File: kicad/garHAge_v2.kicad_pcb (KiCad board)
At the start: 2 copper layers, 99 x 77 mm, 77 parts, among them J1 0813-1X1T-57-F, J2 Serial Interface, J3 SJ1-2503A, J4 SJ1-2503A, J5 SJ1-2503A, J6 SJ1-2503A, J7 SJ1-2503A, J8 SJ1-2503A, K1 G5LE-14_DC3, K2 G5LE-14_DC3, K3 G5LE-14_DC3, Q1 BC846B_215, Q2 BC846B_215, Q3 BC846B_215, U1 ATMEGA328P-AU, U2 NCP1090, U3 PG02S4805A, U4 W5500, U5 LTV-817S, U6 LTV-817S, U7 LTV-817S, X1 ICSP, X2 SPI Disconnect, Y1 8MHz, Y2 25MHz

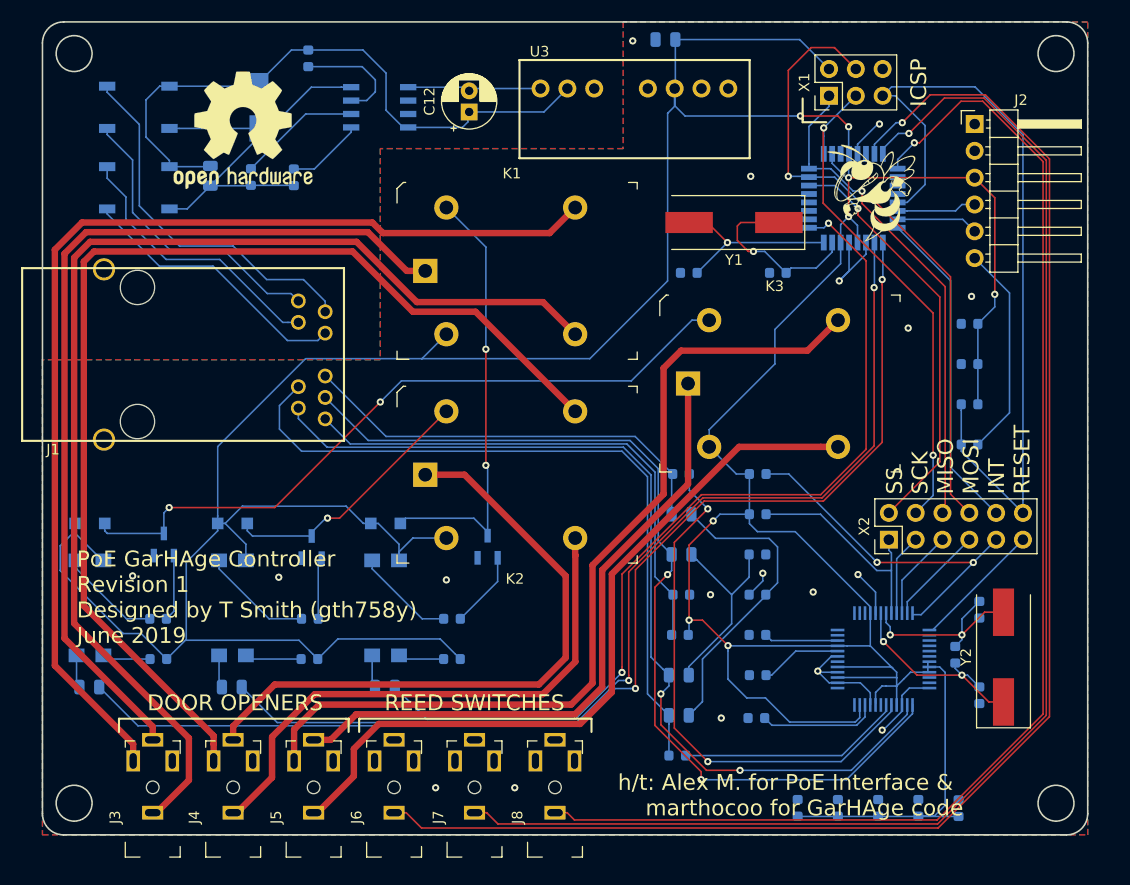
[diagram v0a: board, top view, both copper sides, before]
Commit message: Add files via upload
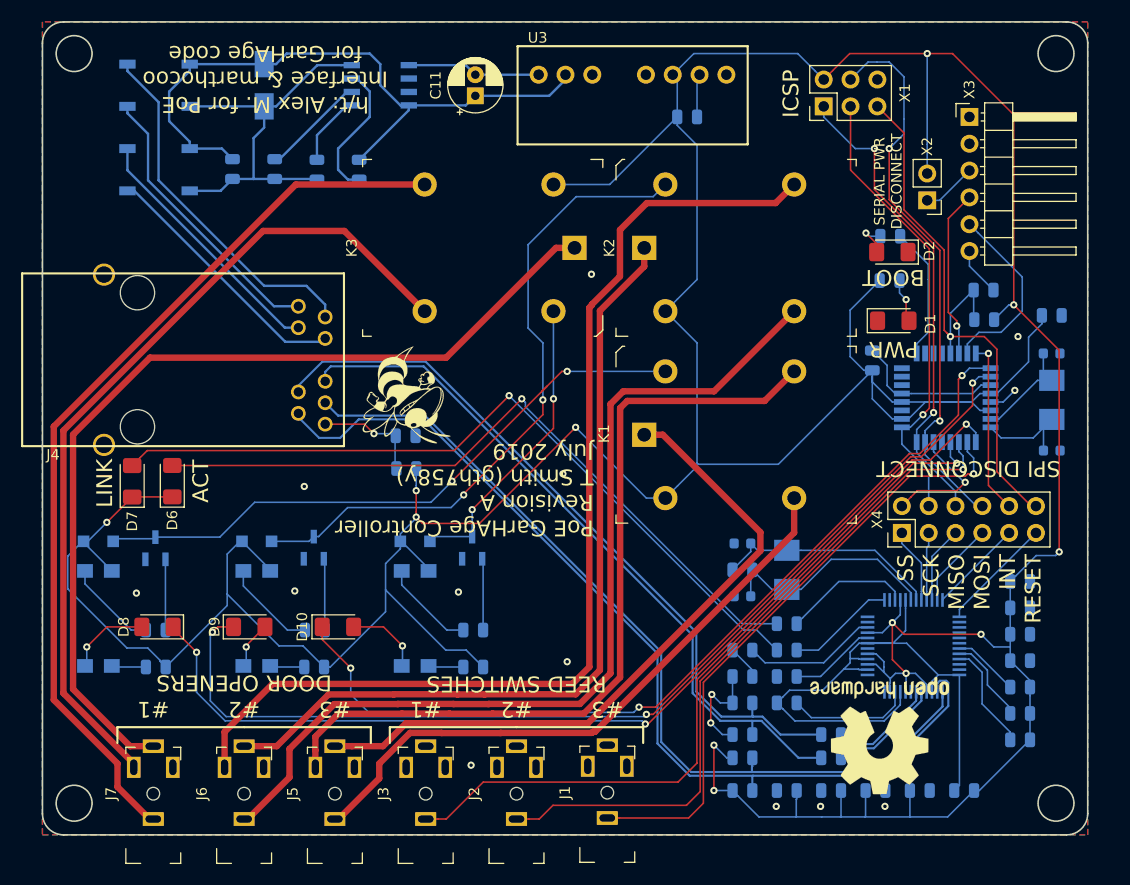
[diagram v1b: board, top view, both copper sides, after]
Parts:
- removed J8: SJ1-2503A, digikey-footprints:Headphone_Jack_2.5mm_SJ1-2503A
- added C23: 4.7u, Capacitor_SMD:C_0805_2012Metric, B.Cu at (191.5, 103.0)
- added C24: 18p, Capacitor_SMD:C_0603_1608Metric, B.Cu at (187.3, 95.4)
- added C25: 18p, Capacitor_SMD:C_0603_1608Metric, B.Cu at (187.3, 90.4)
- added D10: LED, LED_SMD:LED_1206_3216Metric_Pad1.42x1.75mm_HandSolder, F.Cu at (149.0, 98.3)
- added D11: CGRKM4007-HF, Diode_SMD:D_SOD-123F, B.Cu at (126.3, 90.2)
- added D12: CGRKM4007-HF, Diode_SMD:D_SOD-123F, B.Cu at (141.3, 90.2)
- added D13: CGRKM4007-HF, Diode_SMD:D_SOD-123F, B.Cu at (156.3, 90.2)
- added R19: 100, Resistor_SMD:R_0805_2012Metric, B.Cu at (146.7, 102.1)
- added R20: 100, Resistor_SMD:R_0805_2012Metric, B.Cu at (161.8, 102.1)
- added R21: 1k, Resistor_SMD:R_0805_2012Metric, B.Cu at (131.7, 98.6)
- added R22: 1k, Resistor_SMD:R_0805_2012Metric, B.Cu at (146.8, 98.6)
- added R23: 1k, Resistor_SMD:R_0805_2012Metric, B.Cu at (161.8, 98.6)
- added X3: Serial Interface, Connector_PinHeader_2.54mm:PinHeader_1x06_P2.54mm_Horizontal, F.Cu at (208.8, 50.0)
- added X4: SPI Disconnect, Connector_PinHeader_2.54mm:PinHeader_2x06_P2.54mm_Vertical, F.Cu at (202.4, 89.4)
- C1, C2: value 10n -> 6.8n; footprint Capacitor_SMD:C_0603_1608Metric -> Capacitor_SMD:C_0805_2012Metric
- C10, C15, C16, C17, C18, C9, L1: footprint Capacitor_SMD:C_0603_1608Metric -> Capacitor_SMD:C_0805_2012Metric
- C11: value 100n -> 22u; footprint Capacitor_SMD:C_0805_2012Metric -> Capacitor_THT:CP_Radial_D5.0mm_P2.00mm; moved to F.Cu
- C12: value 22u -> 10u; footprint Capacitor_THT:CP_Radial_D5.0mm_P2.00mm -> Capacitor_SMD:C_0805_2012Metric; moved to B.Cu
- C13: value 10u -> 10u/16V
- C14: value 100n -> 10u/16V; footprint Capacitor_SMD:C_0603_1608Metric -> Capacitor_SMD:C_0805_2012Metric
- C19: value 10n -> 100n; footprint Capacitor_SMD:C_0603_1608Metric -> Capacitor_SMD:C_0805_2012Metric
- C20: value 4.7u -> 100n; footprint Capacitor_SMD:C_0603_1608Metric -> Capacitor_SMD:C_0805_2012Metric
- C21, C7, C8: value 18p -> 100n; footprint Capacitor_SMD:C_0603_1608Metric -> Capacitor_SMD:C_0805_2012Metric
- C22: value 18p -> 10n; footprint Capacitor_SMD:C_0603_1608Metric -> Capacitor_SMD:C_0805_2012Metric
- C3: value 100n -> 22n; footprint Capacitor_SMD:C_0603_1608Metric -> Capacitor_SMD:C_0805_2012Metric
- C4: value 100n -> 10n; footprint Capacitor_SMD:C_0603_1608Metric -> Capacitor_SMD:C_0805_2012Metric
- C5, C6: value 100n -> 18p
- D1, D2: value MDB6S -> LED; footprint tyler_components:Micro-DIP-4 -> LED_SMD:LED_1206_3216Metric_Pad1.42x1.75mm_HandSolder; moved to F.Cu
- D3: value SMAJ58A -> MDB6S; footprint Diode_SMD:D_SMA -> tyler_components:Micro-DIP-4
- D4: value LED -> MDB6S; footprint LED_SMD:LED_0805_2012Metric -> tyler_components:Micro-DIP-4
- D5: value LED -> SMAJ58A; footprint LED_SMD:LED_0805_2012Metric -> Diode_SMD:D_SMA
- D6: footprint LED_SMD:LED_0805_2012Metric -> LED_SMD:LED_1206_3216Metric_Pad1.42x1.75mm_HandSolder; moved to F.Cu
- D7, D8, D9: value CGRKM4007-HF -> LED; footprint Diode_SMD:D_SOD-123F -> LED_SMD:LED_1206_3216Metric_Pad1.42x1.75mm_HandSolder; moved to F.Cu
- J1: value 0813-1X1T-57-F -> SJ1-2503A; footprint tyler_components:0813-1X1T-57-F_RJ45-Jack -> digikey-footprints:Headphone_Jack_2.5mm_SJ1-2503A
- J2: value Serial Interface -> SJ1-2503A; footprint Connector_PinHeader_2.54mm:PinHeader_1x06_P2.54mm_Horizontal -> digikey-footprints:Headphone_Jack_2.5mm_SJ1-2503A
- J4: value SJ1-2503A -> 0813-1X1T-57-F; footprint digikey-footprints:Headphone_Jack_2.5mm_SJ1-2503A -> tyler_components:0813-1X1T-57-F_RJ45-Jack
- R10: value 10k -> 4420; footprint Resistor_SMD:R_0603_1608Metric -> Resistor_SMD:R_0805_2012Metric
- R11: footprint Resistor_SMD:R_0603_1608Metric -> Resistor_SMD:R_0805_2012Metric
- R12: value 1M -> 10k; footprint Resistor_SMD:R_0603_1608Metric -> Resistor_SMD:R_0805_2012Metric
- R13: value 1k -> 10k; footprint Resistor_SMD:R_0603_1608Metric -> Resistor_SMD:R_0805_2012Metric
- R14: value 1k -> 12.4k; footprint Resistor_SMD:R_0603_1608Metric -> Resistor_SMD:R_0805_2012Metric
- R15: value 1k -> 1M; footprint Resistor_SMD:R_0603_1608Metric -> Resistor_SMD:R_0805_2012Metric
- R16, R17: value 510 -> 330; footprint Resistor_SMD:R_0603_1608Metric -> Resistor_SMD:R_0805_2012Metric
- R18: value 510 -> 100; footprint Resistor_SMD:R_0603_1608Metric -> Resistor_SMD:R_0805_2012Metric
- R5: value 12k -> 330; footprint Resistor_SMD:R_0603_1608Metric -> Resistor_SMD:R_0805_2012Metric
- R6: value 24.9k -> 12k; footprint Resistor_SMD:R_0603_1608Metric -> Resistor_SMD:R_0805_2012Metric
- R7: value 178k -> 330; footprint Resistor_SMD:R_0603_1608Metric -> Resistor_SMD:R_0805_2012Metric
- R8: value 4420 -> 24.9k; footprint Resistor_SMD:R_0603_1608Metric -> Resistor_SMD:R_0805_2012Metric
- R9: value 12.4k -> 178k; footprint Resistor_SMD:R_0603_1608Metric -> Resistor_SMD:R_0805_2012Metric
- X2: value SPI Disconnect -> Serial Pwr Disconnect; footprint Connector_PinHeader_2.54mm:PinHeader_2x06_P2.54mm_Vertical -> Connector_PinHeader_2.54mm:PinHeader_1x02_P2.54mm_Vertical
- Y1, Y2: footprint Crystal:Crystal_SMD_HC49-SD -> Crystal:Crystal_SMD_5032-2Pin_5.0x3.2mm; moved to B.Cu
- moved REF** 83.2 mm to (200.3, 108.6), turned to 180 degrees
- moved J2 76.9 mm to (165.9, 114.1), turned to 90 degrees
- moved D2 72.7 mm to (201.5, 62.8), turned to 180 degrees
- moved D1 72.6 mm to (201.6, 69.3), turned to 0 degrees
- moved C10 72.2 mm to (139.0, 54.9), turned to 270 degrees
- moved R6 68.6 mm to (210.2, 69.2), turned to 0 degrees
- moved R9 66.6 mm to (147.0, 55.0), turned to 270 degrees
- moved C13 61.3 mm to (213.6, 94.0), turned to 0 degrees
- moved D4 60.9 mm to (132.0, 47.0), turned to 270 degrees
- moved J1 60.8 mm to (174.5, 114.0)
- moved D5 57.1 mm to (142.0, 47.0), turned to 270 degrees
- moved R7 56.8 mm to (201.3, 61.3), turned to 180 degrees
- moved R10 56.2 mm to (143.0, 54.9), turned to 270 degrees
- moved R15 56.0 mm to (187.3, 92.9), turned to 180 degrees
- moved R13 53.9 mm to (213.6, 104.0), turned to 180 degrees
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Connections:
- C1 pad 2: Net-(C1-Pad2) -> /RD-
- C10 pad 1: +3V3 -> Net-(C10-Pad1)
- C10 pad 2: GND -> Net-(C10-Pad2)
- C11 pad 1: Net-(C11-Pad1) -> Net-(C10-Pad1)
- C12 pad 1: Net-(C11-Pad1) -> +3V3
- C12 pad 2: Net-(C12-Pad2) -> GND
- C19 pad 1: Net-(C19-Pad1) -> +3V3
- C2 pad 2: Net-(C2-Pad2) -> /RD+
- C20 pad 1: Net-(C20-Pad1) -> +3V3
- C21 pad 1: GND -> +3V3
- C21 pad 2: Net-(C21-Pad2) -> GND
- C22 pad 1: GND -> Net-(C22-Pad1)
- C22 pad 2: Net-(C22-Pad2) -> GND
- C3 pad 2: Net-(C3-Pad2) -> /CT
- C6 pad 1: DTR -> Net-(C6-Pad1)
- C6 pad 2: RESET -> GND
- C7 pad 1: GND -> DTR
- C7 pad 2: Net-(C7-Pad2) -> RESET
- C8 pad 1: Net-(C8-Pad1) -> +3V3
- D1 pad 1: Net-(C11-Pad1) -> GND
- D1 pad 2: Net-(C11-Pad2) -> Net-(D1-Pad2)
- D2 pad 1: Net-(C11-Pad1) -> GND
- D2 pad 2: Net-(C11-Pad2) -> /BOOT_STATUS
- D3 pad 1: Net-(C11-Pad1) -> Net-(C10-Pad1)
- D3 pad 2: Net-(C11-Pad2) -> Net-(C10-Pad2)
- D4 pad 1: D1RELAY -> Net-(C10-Pad1)
- D4 pad 2: Net-(D4-Pad2) -> Net-(C10-Pad2)
- D5 pad 1: D2RELAY -> Net-(C10-Pad1)
- D5 pad 2: Net-(D5-Pad2) -> Net-(C10-Pad2)
- D6 pad 1: D3RELAY -> +3V3
- D8 pad 1: +3V3 -> D1RELAY
- D9 pad 1: +3V3 -> D2RELAY
- J1 pad 1: /W5100_Ethernet_Interface/TD+ -> D1SENSOR
- J1 pad 2: Net-(C2-Pad2) -> (no net)
- J2 pad 1: GND -> D2SENSOR
- J2 pad 2: GND -> (no net)
- J2 pad 3: +3V3 -> (no net)
- J2 pad 4: RXI -> GND
- J3 pad 1: Net-(J3-Pad1) -> D3SENSOR
- J3 pad 3: Net-(J3-Pad3) -> (no net)
- J3 pad 4: Net-(J3-Pad4) -> GND
- J4 pad 1: Net-(J4-Pad1) -> /W5100_Ethernet_Interface/TD+
- J4 pad 2: (no net) -> /RD+
- J6 pad 3: (no net) -> Net-(J6-Pad3)
- J6 pad 4: GND -> Net-(J6-Pad4)
- J7 pad 3: (no net) -> Net-(J7-Pad3)
- J7 pad 4: GND -> Net-(J7-Pad4)
- K1 pad 1: Net-(J3-Pad4) -> Net-(J5-Pad4)
- K1 pad 3: Net-(J3-Pad1) -> Net-(J5-Pad1)
- K1 pad 4: Net-(J3-Pad3) -> Net-(J5-Pad3)
- K1 pad 5: Net-(D7-Pad2) -> Net-(D11-Pad2)
- K2 pad 1: Net-(J4-Pad4) -> Net-(J6-Pad4)
- K2 pad 3: Net-(J4-Pad1) -> Net-(J6-Pad1)
- K2 pad 4: Net-(J4-Pad3) -> Net-(J6-Pad3)
- K2 pad 5: Net-(D8-Pad2) -> Net-(D12-Pad2)
- K3 pad 1: Net-(J5-Pad4) -> Net-(J7-Pad4)
- K3 pad 3: Net-(J5-Pad1) -> Net-(J7-Pad1)
- K3 pad 4: Net-(J5-Pad3) -> Net-(J7-Pad3)
- K3 pad 5: Net-(D9-Pad2) -> Net-(D13-Pad2)
- L1 pad 2: Net-(C3-Pad2) -> /CT
- Q1 pad 3: Net-(D7-Pad2) -> Net-(D11-Pad2)
- Q2 pad 3: Net-(D8-Pad2) -> Net-(D12-Pad2)
- Q3 pad 3: Net-(D9-Pad2) -> Net-(D13-Pad2)
- R1 pad 1: Net-(C4-Pad2) -> +3V3
- R10 pad 1: +3V3 -> Net-(R10-Pad1)
- R10 pad 2: W_CS -> Net-(C10-Pad2)
- R11 pad 1: W_INT -> +3V3
- R11 pad 2: +3V3 -> Net-(R11-Pad2)
- R12 pad 1: Net-(C21-Pad2) -> +3V3
- R12 pad 2: Net-(C22-Pad2) -> Net-(R12-Pad2)
- R13 pad 1: Net-(R13-Pad1) -> +3V3
- R13 pad 2: +3V3 -> Net-(R13-Pad2)
- R14 pad 1: Net-(R14-Pad1) -> GND
- R14 pad 2: +3V3 -> Net-(R14-Pad2)
- R15 pad 1: Net-(R15-Pad1) -> Net-(C24-Pad2)
- R15 pad 2: +3V3 -> Net-(C25-Pad2)
- R16 pad 1: Net-(Q1-Pad1) -> Net-(D6-Pad2)
- R17 pad 1: Net-(Q2-Pad1) -> Net-(D7-Pad2)
- R18 pad 1: Net-(Q3-Pad1) -> Net-(R18-Pad1)
- R18 pad 2: Net-(R18-Pad2) -> +3V3
- R2 pad 1: Net-(C4-Pad2) -> +3V3
- R3 pad 1: Net-(C5-Pad2) -> Net-(C4-Pad2)
- R3 pad 2: Net-(C2-Pad2) -> /RD+
- R4 pad 1: Net-(C5-Pad2) -> Net-(C4-Pad2)
- R4 pad 2: Net-(C1-Pad2) -> /RD-
- R5 pad 1: RESET -> Net-(D1-Pad2)
- R6 pad 1: Net-(C11-Pad1) -> RESET
- R6 pad 2: Net-(R6-Pad2) -> +3V3
- R7 pad 2: Net-(C11-Pad2) -> /BOOT_STATUS
- R8 pad 1: Net-(R8-Pad1) -> Net-(C10-Pad1)
- R8 pad 2: Net-(C11-Pad2) -> Net-(R8-Pad2)
- R9 pad 1: GND -> Net-(R9-Pad1)
- R9 pad 2: Net-(R9-Pad2) -> Net-(C10-Pad2)
- U1 pad 10: (no net) -> D1SENSOR
- U1 pad 11: (no net) -> D2SENSOR
- U1 pad 12: (no net) -> D3SENSOR
- U1 pad 23: Net-(J6-Pad1) -> (no net)
- U1 pad 24: Net-(J7-Pad1) -> (no net)
- U1 pad 25: Net-(J8-Pad1) -> Net-(R7-Pad1)
- U1 pad 7: Net-(C7-Pad2) -> Net-(C5-Pad2)
- U1 pad 8: Net-(C8-Pad1) -> Net-(C6-Pad1)
- U2 pad 1: Net-(R7-Pad1) -> Net-(R9-Pad1)
- U2 pad 2: Net-(R8-Pad1) -> Net-(R10-Pad1)
- U2 pad 3: Net-(R6-Pad2) -> Net-(R8-Pad2)
- U2 pad 4: Net-(C11-Pad2) -> Net-(C10-Pad2)
- U2 pad 5: Net-(C12-Pad2) -> Net-(C11-Pad2)
- U2 pad 8: Net-(C11-Pad1) -> Net-(C10-Pad1)
- U3 pad 1: Net-(C12-Pad2) -> Net-(C11-Pad2)
- U3 pad 2: Net-(C11-Pad1) -> Net-(C10-Pad1)
- U4 pad 10: Net-(R9-Pad2) -> Net-(R14-Pad2)
- U4 pad 20: Net-(C20-Pad1) -> Net-(C23-Pad1)
- U4 pad 22: Net-(C19-Pad1) -> Net-(C22-Pad1)
- U4 pad 25: (no net) -> Net-(R17-Pad2)
- U4 pad 27: (no net) -> Net-(R16-Pad2)
- U4 pad 30: Net-(C21-Pad2) -> Net-(C24-Pad2)
- U4 pad 31: Net-(C22-Pad2) -> Net-(C25-Pad2)
- U4 pad 43: +3V3 -> Net-(R13-Pad2)
- U4 pad 44: +3V3 -> Net-(R12-Pad2)
- U4 pad 45: +3V3 -> Net-(R11-Pad2)
- U5 pad 1: Net-(R13-Pad1) -> Net-(R18-Pad1)
- U5 pad 2: Net-(D4-Pad2) -> Net-(D8-Pad2)
- U5 pad 3: Net-(R16-Pad2) -> Net-(R21-Pad2)
- U6 pad 1: Net-(R14-Pad1) -> Net-(R19-Pad1)
- U6 pad 2: Net-(D5-Pad2) -> Net-(D9-Pad2)
- U6 pad 3: Net-(R17-Pad2) -> Net-(R22-Pad2)
- U7 pad 1: Net-(R15-Pad1) -> Net-(R20-Pad1)
- U7 pad 2: Net-(D6-Pad2) -> Net-(D10-Pad2)
- U7 pad 3: Net-(R18-Pad2) -> Net-(R23-Pad2)
- X2 pad 1: W_CS -> Net-(X2-Pad1)
- X2 pad 2: SS -> +3V3
- Y1 pad 1: Net-(C7-Pad2) -> Net-(C5-Pad2)
- Y1 pad 2: Net-(C8-Pad1) -> Net-(C6-Pad1)
- Y2 pad 1: Net-(C21-Pad2) -> Net-(C24-Pad2)
- Y2 pad 2: Net-(C22-Pad2) -> Net-(C25-Pad2)
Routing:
- net Net-(J8-Pad1): track 122.3 -> 0.00 mm, vias 1 -> 0
- net Net-(J3-Pad1): track 110.4 -> 0.00 mm
- net Net-(J4-Pad3): track 105.6 -> 0.00 mm
- net Net-(J3-Pad3): track 103.3 -> 0.00 mm
- net Net-(J6-Pad3): track 0.00 -> 101.3 mm
- net Net-(J7-Pad4): track 0.00 -> 88.8 mm
- net Net-(J3-Pad4): track 86.0 -> 0.00 mm
- net Net-(J7-Pad3): track 0.00 -> 79.8 mm
- net Net-(J6-Pad4): track 0.00 -> 78.4 mm
- net D3SENSOR: track 0.00 -> 71.1 mm, vias 0 -> 1
- net /RD+: track 0.00 -> 70.3 mm
- net Net-(C2-Pad2): track 68.7 -> 0.00 mm
- net /RD-: track 0.00 -> 68.0 mm
- net Net-(D6-Pad2): track 3.11 -> 68.9 mm, vias 0 -> 1
- net D2SENSOR: track 0.00 -> 64.9 mm, vias 0 -> 1
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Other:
- net class 48V Handling added: clearance 0.1524, trace_width 0.2286, via_dia 0.6858, via_drill 0.3302
- net class Diff Pairs added: clearance 0.1524, trace_width 0.2, via_dia 0.6858, via_drill 0.3302
- board text added: "#1"
- board text added: "#2"
- board text added: "#3"
- board text added: "ACT"
- board text added: "BOOT"
- board text added: "LINK"
- board text added: "PWR"
- board text added: "PoE GarHAge Controller Revision A T Smith (gth758y) July 2019"
- board text added: "SERIAL PWR DISCONNECT"
- board text added: "SPI DISCONNECT"
- board text added: "Serial Debug"
- board text removed: "PoE GarHAge Controller Revision 1 Designed by T Smith (gth758y) June 2019"
- board text removed: "SERIAL DEBUG"
